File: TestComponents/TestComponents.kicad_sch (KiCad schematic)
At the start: 18 parts, among them J3V1 Conn_01x01_Male, J5 RFShield_OnePiece, J6 RFShield_OnePiece, U1 AD7991, U2 ADS1219

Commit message: SpectDrone Development
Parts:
- C15, C38: Part Number CL05C2R5CB5NNNC -> CQ0402ARNPO9BN2R5
- U2: Part Number ADS1219 -> ADS1219IPWR
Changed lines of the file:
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@@
       (effects (font (size 1.27 1.27)) hide)
     )
-    (property "Part Number" "CL05C2R5CB5NNNC" (id 4) (at 33.02 35.56 0)
+    (property "Part Number" "CQ0402ARNPO9BN2R5" (id 4) (at 33.02 35.56 0)
       (effects (font (size 1.27 1.27)) hide)
     )
@@
       (effects (font (size 1.27 1.27)) hide)
     )
-    (property "Part Number" "CL05C2R5CB5NNNC" (id 4) (at 111.76 35.56 0)
+    (property "Part Number" "CQ0402ARNPO9BN2R5" (id 4) (at 111.76 35.56 0)
       (effects (font (size 1.27 1.27)) hide)
     )
@@
       (effects (font (size 1.27 1.27)) hide)
     )
-    (property "Part Number" "ADS1219" (id 4) (at 72.39 46.99 0)
+    (property "Part Number" "ADS1219IPWR" (id 4) (at 72.39 46.99 0)
       (effects (font (size 1.27 1.27)) hide)
     )

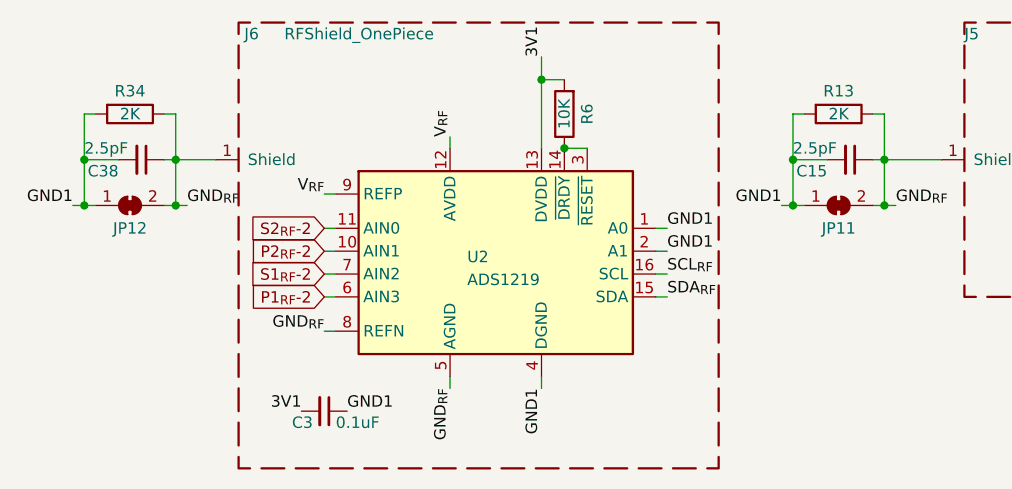
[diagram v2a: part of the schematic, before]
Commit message: SpectDrone Development
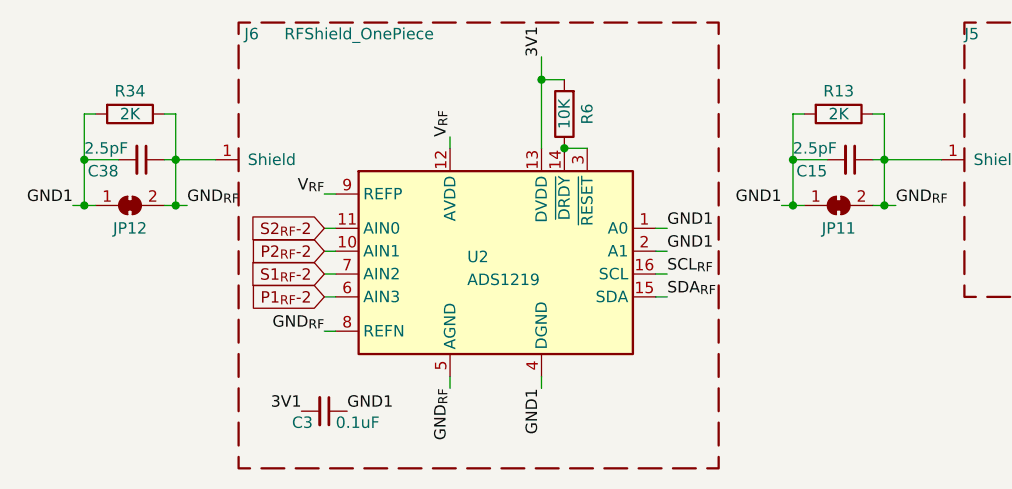
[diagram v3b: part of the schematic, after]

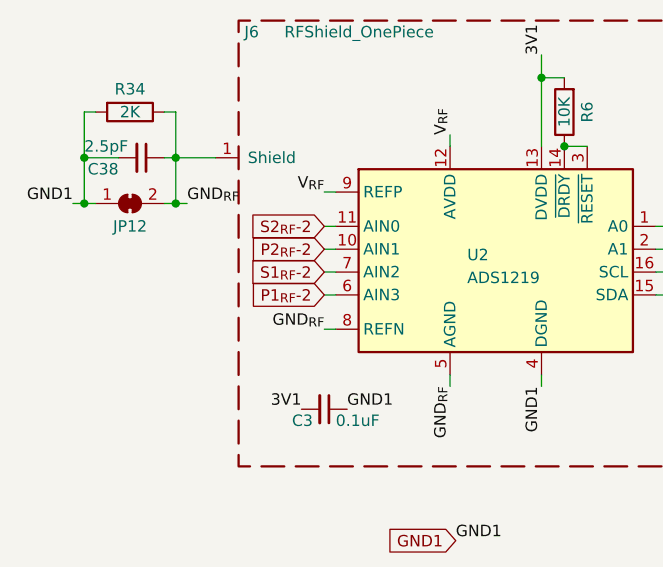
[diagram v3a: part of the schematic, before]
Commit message: SpectDrone Development
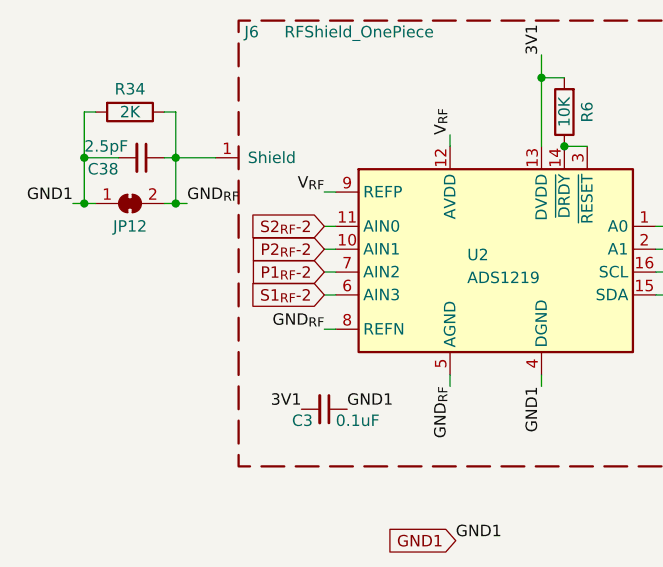
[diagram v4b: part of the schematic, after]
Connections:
- net P1_{RF}-2: now also U2.7 (AIN2); no longer U2.6 (AIN3)
- net S1_{RF}-2: now also U2.6 (AIN3); no longer U2.7 (AIN2)
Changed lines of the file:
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@@
     )
   )
-  (global_label "S1_{RF}-2" (shape input) (at 53.34 48.26 180) (fields_autoplaced)
+  (global_label "S1_{RF}-2" (shape input) (at 53.34 50.8 180) (fields_autoplaced)
     (effects (font (size 1.27 1.27)) (justify right))
-    (property "Intersheetrefs" "${INTERSHEET_REFS}" (at 43.8391 48.1806 0)
+    (property "Intersheetrefs" "${INTERSHEET_REFS}" (at 43.8391 50.8794 0)
       (effects (font (size 1.27 1.27)) (justify right) hide)
     )
@@
     )
   )
-  (global_label "P1_{RF}-2" (shape input) (at 53.34 50.8 180) (fields_autoplaced)
+  (global_label "P1_{RF}-2" (shape input) (at 53.34 48.26 180) (fields_autoplaced)
     (effects (font (size 1.27 1.27)) (justify right))
-    (property "Intersheetrefs" "${INTERSHEET_REFS}" (at 43.7786 50.7206 0)
+    (property "Intersheetrefs" "${INTERSHEET_REFS}" (at 43.7786 48.3394 0)
       (effects (font (size 1.27 1.27)) (justify right) hide)
     )

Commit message: SpectDrone Development
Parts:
- J3V1, JVIN1: now left out of the parts list
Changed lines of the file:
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@@
   )
   (symbol (lib_id "Connector:Conn_01x01_Male") (at 126.365 106.045 0) (unit 1)
-    (in_bom yes) (on_board yes) (dnp no) (fields_autoplaced)
+    (in_bom no) (on_board yes) (dnp no) (fields_autoplaced)
     (property "Reference" "J3V1" (at 127 100.33 0)
       (effects (font (size 1.27 1.27)))
@@
   )
   (symbol (lib_id "Connector:Conn_01x01_Male") (at 126.365 114.3 0) (unit 1)
-    (in_bom yes) (on_board yes) (dnp no) (fields_autoplaced)
+    (in_bom no) (on_board yes) (dnp no) (fields_autoplaced)
     (property "Reference" "JVIN1" (at 127 109.22 0)
       (effects (font (size 1.27 1.27)))

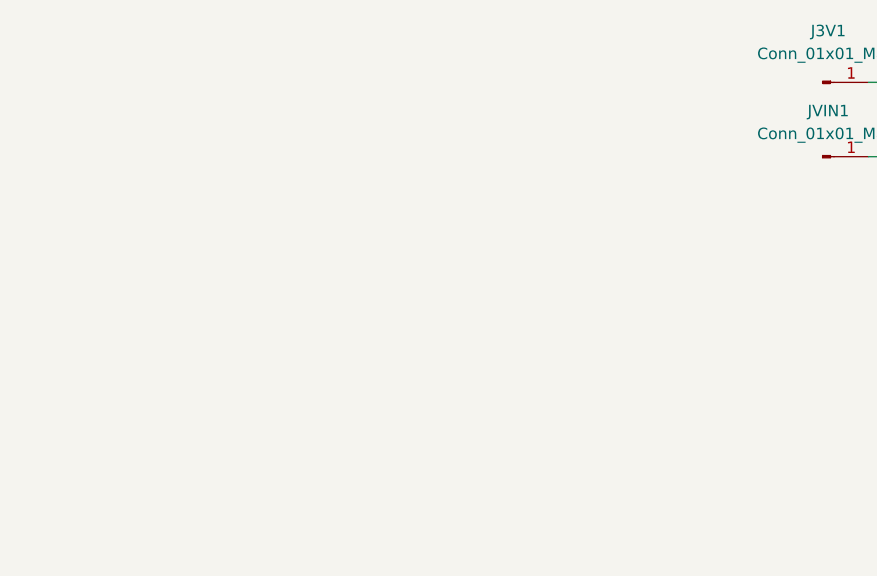
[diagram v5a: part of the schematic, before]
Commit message: SpectDrone Development
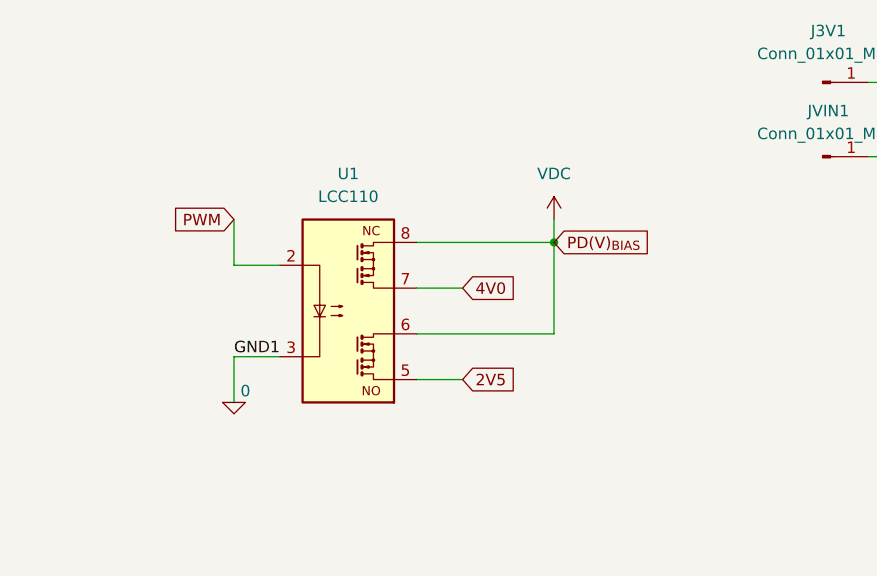
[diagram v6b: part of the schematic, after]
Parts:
- added U1: LCC110, Package_DIP:DIP-8_W8.89mm_SMDSocket_LongPads, symbol Relay_SolidState:LCC110
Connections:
- net GND1 renamed 0
- net 0: now also U1.3
- new net 2V5: U1.5
- new net 4V0: U1.7
- new net PWM: U1.2
- new net VDC: U1.6, U1.8
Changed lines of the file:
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@@
   (junction (at 171.45 33.02) (diameter 0) (color 0 0 0 0)
   )
+  (junction (at 96.52 123.825) (diameter 0) (color 0 0 0 0)
+  )
   (junction (at 26.67 40.64) (diameter 0) (color 0 0 0 0)
   )
@@
     (stroke (width 0) (type default))
   )
+  (wire (pts (xy 60.96 136.525) (xy 66.04 136.525))
+    (stroke (width 0) (type default))
+  )
   (wire (pts (xy 105.41 30.48) (xy 105.41 35.56))
     (stroke (width 0) (type default))
@@
     (stroke (width 0) (type default))
   )
+  (wire (pts (xy 66.04 126.365) (xy 60.96 126.365))
+    (stroke (width 0) (type default))
+  )
   (wire (pts (xy 106.68 30.48) (xy 105.41 30.48))
     (stroke (width 0) (type default))
@@
     (stroke (width 0) (type default))
   )
+  (wire (pts (xy 60.96 121.285) (xy 60.96 126.365))
+    (stroke (width 0) (type default))
+  )
   (wire (pts (xy 189.23 28.575) (xy 197.485 28.575))
     (stroke (width 0) (type default))
@@
     (stroke (width 0) (type default))
   )
+  (wire (pts (xy 81.28 128.905) (xy 86.36 128.905))
+    (stroke (width 0) (type default))
+  )
   (wire (pts (xy 36.83 40.64) (xy 38.1 40.64))
     (stroke (width 0) (type default))
@@
     (stroke (width 0) (type default))
   )
+  (wire (pts (xy 81.28 133.985) (xy 96.52 133.985))
+    (stroke (width 0) (type default))
+  )
   (wire (pts (xy 157.48 39.37) (xy 158.115 38.735))
     (stroke (width 0) (type default))
@@
     (stroke (width 0) (type default))
   )
+  (wire (pts (xy 96.52 121.285) (xy 96.52 123.825))
+    (stroke (width 0) (type default))
+  )
   (wire (pts (xy 135.255 33.02) (xy 142.24 33.02))
     (stroke (width 0) (type default))
@@
     (stroke (width 0) (type default))
   )
+  (wire (pts (xy 60.96 141.605) (xy 60.96 136.525))
+    (stroke (width 0) (type default))
+  )
   (wire (pts (xy 53.34 48.26) (xy 54.61 48.26))
     (stroke (width 0) (type default))
@@
     (stroke (width 0) (type default))
   )
+  (wire (pts (xy 81.28 139.065) (xy 86.36 139.065))
+    (stroke (width 0) (type default))
+  )
   (wire (pts (xy 91.44 50.8) (xy 90.17 50.8))
     (stroke (width 0) (type default))
   )
+  (wire (pts (xy 96.52 123.825) (xy 96.52 133.985))
+    (stroke (width 0) (type default))
+  )
   (wire (pts (xy 26.67 35.56) (xy 26.67 40.64))
     (stroke (width 0) (type default))
@@
     (stroke (width 0) (type default))
   )
+  (wire (pts (xy 81.28 123.825) (xy 96.52 123.825))
+    (stroke (width 0) (type default))
+  )
   (wire (pts (xy 77.47 24.13) (xy 77.47 26.67))
     (stroke (width 0) (type default))
@@
     (effects (font (size 1.27 1.27)) (justify left bottom))
   )
+  (label "GND1" (at 60.96 136.525 0) (fields_autoplaced)
+    (effects (font (size 1.27 1.27)) (justify left bottom))
+  )
   (label "SCL_{RF}" (at 91.44 48.26 0) (fields_autoplaced)
     (effects (font (size 1.27 1.27)) (justify left bottom))
@@
     )
   )
+  (global_label "PWM" (shape input) (at 60.96 121.285 180) (fields_autoplaced)
+    (effects (font (size 1.27 1.27)) (justify right))
+    (property "Intersheetrefs" "${INTERSHEET_REFS}" (at 53.802 121.285 0)
+      (effects (font (size 1.27 1.27)) (justify right) hide)
+    )
+  )
   (global_label "3V1" (shape input) (at 137.16 106.045 0) (fields_autoplaced)
     (effects (font (size 1.27 1.27)) (justify left))
@@
     )
   )
+  (global_label "PD(V)_{BIAS}" (shape input) (at 96.52 123.825 0) (fields_autoplaced)
+    (effects (font (size 1.27 1.27)) (justify left))
+    (property "Intersheetrefs" "${INTERSHEET_REFS}" (at 108.2163 123.825 0)
+      (effects (font (size 1.27 1.27)) (justify left) hide)
+    )
+  )
   (global_label "VIN" (shape input) (at 137.16 114.3 0) (fields_autoplaced)
     (effects (font (size 1.27 1.27)) (justify left))
@@
     )
   )
+  (global_label "4V0" (shape input) (at 86.36 128.905 0) (fields_autoplaced)
+    (effects (font (size 1.27 1.27)) (justify left))
+    (property "Intersheetrefs" "${INTERSHEET_REFS}" (at 92.8528 128.905 0)
+      (effects (font (size 1.27 1.27)) (justify left) hide)
+    )
+  )
   (global_label "P2_{RF}" (shape input) (at 207.01 105.41 0) (fields_autoplaced)
     (effects (font (size 1.27 1.27)) (justify left))
@@
     (property "Intersheetrefs" "${INTERSHEET_REFS}" (at 134.8255 42.4656 0)
       (effects (font (size 1.27 1.27)) (justify right) hide)
+    )
+  )
+  (global_label "2V5" (shape input) (at 86.36 139.065 0) (fields_autoplaced)
+    (effects (font (size 1.27 1.27)) (justify left))
+    (property "Intersheetrefs" "${INTERSHEET_REFS}" (at 92.8528 139.065 0)
+      (effects (font (size 1.27 1.27)) (justify left) hide)
     )
   )
@@
     )
   )
+  (symbol (lib_id "Relay_SolidState:LCC110") (at 73.66 131.445 0) (unit 1)
+    (in_bom yes) (on_board yes) (dnp no) (fields_autoplaced)
+    (property "Reference" "U1" (at 73.66 116.205 0)
+      (effects (font (size 1.27 1.27)))
+    )
+    (property "Value" "LCC110" (at 73.66 118.745 0)
+      (effects (font (size 1.27 1.27)))
+    )
+    (property "Footprint" "Package_DIP:DIP-8_W8.89mm_SMDSocket_LongPads" (at 73.66 144.145 0)
+      (effects (font (size 1.27 1.27) italic) hide)
+    )
+    (property "Datasheet" "http://www.ixysic.com/home/pdfs.nsf/www/LCC110.pdf/$file/LCC110.pdf" (at 73.66 131.445 0)
+      (effects (font (size 1.27 1.27)) (justify left) hide)
+    )
+    (pin "1")
+    (pin "2")
+    (pin "3")
+    (pin "4")
+    (pin "5")
+    (pin "6")
+    (pin "7")
+    (pin "8")
+    (instances
+      (project "Mosfet inverting switch"
+        (path "/9f97d8ac-cfa1-49b7-8da4-4ee5ae95f9bd"
+          (reference "U1") (unit 1)
+        )
+      )
+      (project "TestComponents"
+        (path "/e63e39d7-6ac0-4ffd-8aa3-1841a4541b55"
+          (reference "U5") (unit 1)
+        )
+      )
+    )
+  )
   (symbol (lib_id "Device:C_Polarized_Small_US") (at 197.485 34.29 0) (unit 1)
     (in_bom yes) (on_board yes) (dnp no)
@@
         (path "/e63e39d7-6ac0-4ffd-8aa3-1841a4541b55"
           (reference "C1") (unit 1)
+        )
+      )
+    )
+  )
+  (symbol (lib_id "power:VDC") (at 96.52 121.285 0) (unit 1)
+    (in_bom yes) (on_board yes) (dnp no) (fields_autoplaced)
+    (property "Reference" "#PWR01" (at 96.52 123.825 0)
+      (effects (font (size 1.27 1.27)) hide)
+    )
+    (property "Value" "VDC" (at 96.52 116.205 0)
+      (effects (font (size 1.27 1.27)))
+    )
+    (property "Footprint" "" (at 96.52 121.285 0)
+      (effects (font (size 1.27 1.27)) hide)
+    )
+    (property "Datasheet" "" (at 96.52 121.285 0)
+      (effects (font (size 1.27 1.27)) hide)
+    )
+    (pin "1")
+    (instances
+      (project "Mosfet inverting switch"
+        (path "/9f97d8ac-cfa1-49b7-8da4-4ee5ae95f9bd"
+          (reference "#PWR01") (unit 1)
+        )
+      )
+      (project "TestComponents"
+        (path "/e63e39d7-6ac0-4ffd-8aa3-1841a4541b55"
+          (reference "#PWR01") (unit 1)
         )
       )
@@
         )
       )
+    )
+  )
+  (symbol (lib_id "Simulation_SPICE:0") (at 60.96 141.605 0) (unit 1)
+    (in_bom yes) (on_board yes) (dnp no)
+    (property "Reference" "#GND04" (at 60.96 144.145 0)
+      (effects (font (size 1.27 1.27)) hide)
+    )
+    (property "Value" "0" (at 62.23 140.335 0)
+      (effects (font (size 1.27 1.27)))
+    )
+    (property "Footprint" "" (at 60.96 141.605 0)
+      (effects (font (size 1.27 1.27)) hide)
+    )
+    (property "Datasheet" "~" (at 60.96 141.605 0)
+      (effects (font (size 1.27 1.27)) hide)
+    )
+    (pin "1")
+    (instances
+      (project "Mosfet inverting switch"
+        (path "/9f97d8ac-cfa1-49b7-8da4-4ee5ae95f9bd"
+          (reference "#GND04") (unit 1)
+        )
+      )
+      (project "TestComponents"
+        (path "/e63e39d7-6ac0-4ffd-8aa3-1841a4541b55"
+          (reference "#GND01") (unit 1)
+        )
+      )
